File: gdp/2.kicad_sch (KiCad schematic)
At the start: 9 parts, among them IC1 74LS85, IC17 MK3881, IC7 PAL16L8

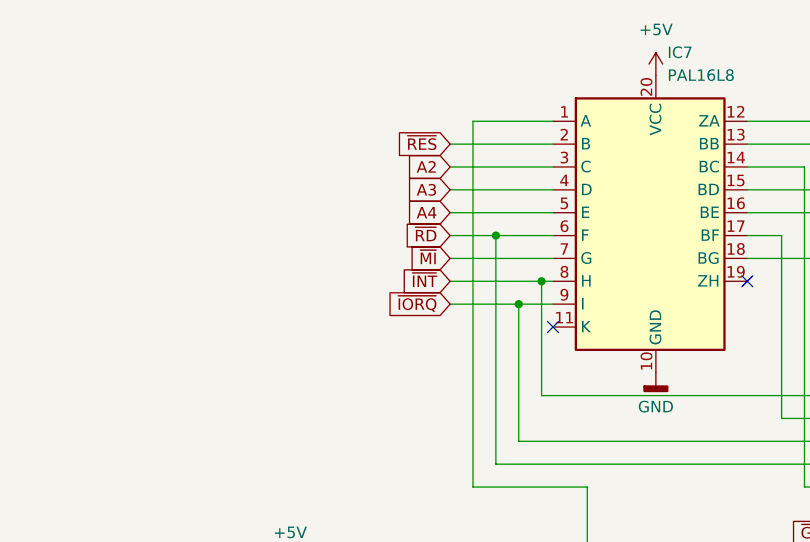
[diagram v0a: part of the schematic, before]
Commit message: Adds Sheet 14 (WIP)
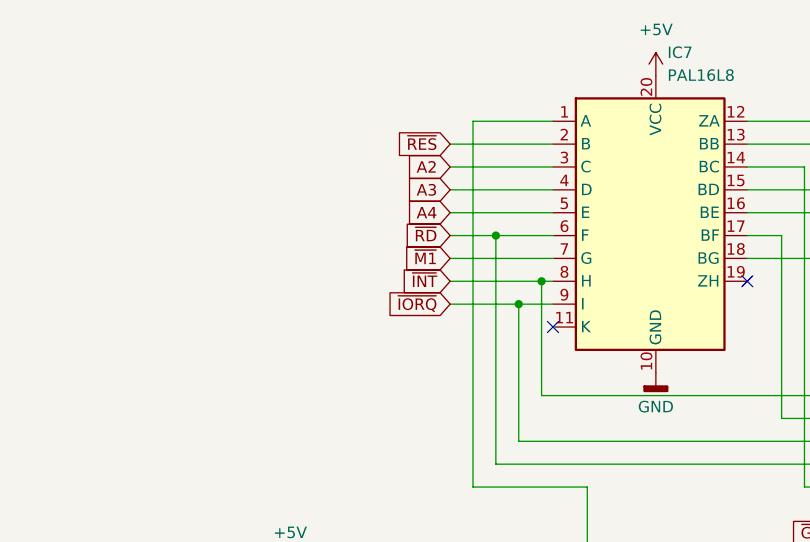
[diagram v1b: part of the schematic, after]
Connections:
- net ~{MI} renamed ~{M1}
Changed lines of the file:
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@@
 		)
 	)
-	(global_label "~{MI}"
+	(global_label "~{M1}"
 		(shape input)
 		(at 115.57 67.31 180)
@@
 		)
 		(property "Intersheetrefs" "${INTERSHEET_REFS}"
-			(at 110.5286 67.31 0)
+			(at 109.9239 67.31 0)
 			(effects
 				(font

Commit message: Initial footprint assignment
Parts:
- IC1: footprint (none) -> Package_DIP:DIP-16_W7.62mm
- IC17: footprint (none) -> Package_DIP:DIP-40_W15.24mm
- IC7: footprint (none) -> Package_DIP:DIP-20_W7.62mm
- R18, R19, R20: footprint (none) -> Resistor_THT:R_Axial_DIN0207_L6.3mm_D2.5mm_P7.62mm_Horizontal
- SH7, SH8, SH9: value SCHALT1 -> SCHALT; footprint (none) -> Connector_PinHeader_2.54mm:PinHeader_1x02_P2.54mm_Vertical
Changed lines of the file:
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@@
 			)
 		)
-		(property "Footprint" ""
+		(property "Footprint" "Resistor_THT:R_Axial_DIN0207_L6.3mm_D2.5mm_P7.62mm_Horizontal"
 			(at 71.12 136.398 90)
 			(effects
@@
 			)
 		)
-		(property "Datasheet" "~"
+		(property "Datasheet" "N/A"
 			(at 71.12 134.62 0)
 			(effects
@@
 			)
 		)
-		(property "Description" ""
+		(property "Description" "N/A"
 			(at 71.12 134.62 0)
 			(effects
@@
 			(project "gdp"
 				(path "/95aff260-2720-4733-a81d-a7a2136fdd14/ed2e3011-1fbf-423e-aa8b-2b4bbe99b1f1"
-					(reference "R18")
+					(reference "R11")
 					(unit 1)
 				)
@@
 		(dnp no)
 		(fields_autoplaced yes)
-		(property "Reference" "#PWR065"
+		(property "Reference" "#PWR032"
 			(at 187.96 144.78 0)
 			(effects
@@
 			(project "gdp"
 				(path "/95aff260-2720-4733-a81d-a7a2136fdd14/ed2e3011-1fbf-423e-aa8b-2b4bbe99b1f1"
-					(reference "#PWR065")
+					(reference "#PWR032")
 					(unit 1)
 				)
@@
 		(dnp no)
 		(fields_autoplaced yes)
-		(property "Reference" "#PWR082"
+		(property "Reference" "#PWR027"
 			(at 114.3 115.57 0)
 			(effects
@@
 			(project "gdp"
 				(path "/95aff260-2720-4733-a81d-a7a2136fdd14/ed2e3011-1fbf-423e-aa8b-2b4bbe99b1f1"
-					(reference "#PWR082")
+					(reference "#PWR027")
 					(unit 1)
 				)
@@
 		(dnp no)
 		(fields_autoplaced yes)
-		(property "Reference" "#PWR064"
+		(property "Reference" "#PWR028"
 			(at 114.3 157.48 0)
 			(effects
@@
 			(project "gdp"
 				(path "/95aff260-2720-4733-a81d-a7a2136fdd14/ed2e3011-1fbf-423e-aa8b-2b4bbe99b1f1"
-					(reference "#PWR064")
+					(reference "#PWR028")
 					(unit 1)
 				)
@@
 			)
 		)
-		(property "Footprint" ""
+		(property "Footprint" "Resistor_THT:R_Axial_DIN0207_L6.3mm_D2.5mm_P7.62mm_Horizontal"
 			(at 71.12 138.938 90)
 			(effects
@@
 			)
 		)
-		(property "Datasheet" "~"
+		(property "Datasheet" "N/A"
 			(at 71.12 137.16 0)
 			(effects
@@
 			)
 		)
-		(property "Description" ""
+		(property "Description" "N/A"
 			(at 71.12 137.16 0)
 			(effects
@@
 			(project "gdp"
 				(path "/95aff260-2720-4733-a81d-a7a2136fdd14/ed2e3011-1fbf-423e-aa8b-2b4bbe99b1f1"
-					(reference "R20")
+					(reference "R12")
 					(unit 1)
 				)
@@
 			)
 		)
-		(property "Footprint" ""
+		(property "Footprint" "Package_DIP:DIP-20_W7.62mm"
 			(at 137.16 41.91 0)
 			(effects
@@
 			)
 		)
-		(property "Datasheet" ""
+		(property "Datasheet" "N/A"
 			(at 137.16 41.91 0)
 			(effects
@@
 			)
 		)
-		(property "Description" ""
+		(property "Description" "N/A"
 			(at 138.43 45.72 0)
 			(effects
@@
 			(project "gdp"
 				(path "/95aff260-2720-4733-a81d-a7a2136fdd14/ed2e3011-1fbf-423e-aa8b-2b4bbe99b1f1"
-					(reference "IC7")
+					(reference "IC5")
 					(unit 1)
 				)
@@
 		(dnp no)
 		(fields_autoplaced yes)
-		(property "Reference" "#PWR074"
+		(property "Reference" "#PWR029"
 			(at 138.43 50.8 0)
 			(effects
@@
 			(project ""
 				(path "/95aff260-2720-4733-a81d-a7a2136fdd14/ed2e3011-1fbf-423e-aa8b-2b4bbe99b1f1"
-					(reference "#PWR074")
+					(reference "#PWR029")
 					(unit 1)
 				)
@@
 			(project "gdp"
 				(path "/95aff260-2720-4733-a81d-a7a2136fdd14/ed2e3011-1fbf-423e-aa8b-2b4bbe99b1f1"
-					(reference "#PWR01")
+					(reference "#PWR025")
 					(unit 1)
 				)
@@
 		(dnp no)
 		(fields_autoplaced yes)
-		(property "Reference" "#PWR063"
+		(property "Reference" "#PWR024"
 			(at 67.31 147.32 0)
 			(effects
@@
 			(project ""
 				(path "/95aff260-2720-4733-a81d-a7a2136fdd14/ed2e3011-1fbf-423e-aa8b-2b4bbe99b1f1"
-					(reference "#PWR063")
+					(reference "#PWR024")
 					(unit 1)
 				)
@@
 		(dnp no)
 		(fields_autoplaced yes)
-		(property "Reference" "#PWR066"
+		(property "Reference" "#PWR030"
 			(at 138.43 86.36 0)
 			(effects
@@
 			(project "gdp"
 				(path "/95aff260-2720-4733-a81d-a7a2136fdd14/ed2e3011-1fbf-423e-aa8b-2b4bbe99b1f1"
-					(reference "#PWR066")
+					(reference "#PWR030")
 					(unit 1)
 				)
@@
 			)
 		)
-		(property "Value" "SCHALT1"
+		(property "Value" "SCHALT"
 			(at 80.01 109.22 0)
 			(effects
@@
 			)
 		)
-		(property "Footprint" ""
+		(property "Footprint" "Connector_PinHeader_2.54mm:PinHeader_1x02_P2.54mm_Vertical"
 			(at 81.28 113.03 0)
 			(effects
@@
 			)
 		)
-		(property "Datasheet" "~"
+		(property "Datasheet" "N/A"
 			(at 81.28 113.03 0)
 			(effects
@@
 			)
 		)
-		(property "Description" ""
+		(property "Description" "N/A"
 			(at 81.28 113.03 0)
 			(effects
@@
 			(project "gdp"
 				(path "/95aff260-2720-4733-a81d-a7a2136fdd14/ed2e3011-1fbf-423e-aa8b-2b4bbe99b1f1"
-					(reference "SH8")
+					(reference "SH5")
 					(unit 1)
 				)
@@
 		(dnp no)
 		(fields_autoplaced yes)
-		(property "Reference" "#PWR075"
+		(property "Reference" "#PWR031"
 			(at 187.96 83.82 0)
 			(effects
@@
 			(project ""
 				(path "/95aff260-2720-4733-a81d-a7a2136fdd14/ed2e3011-1fbf-423e-aa8b-2b4bbe99b1f1"
-					(reference "#PWR075")
+					(reference "#PWR031")
 					(unit 1)
 				)
@@
 			)
 		)
-		(property "Value" "SCHALT1"
+		(property "Value" "SCHALT"
 			(at 77.47 109.22 0)
 			(effects
@@
 			)
 		)
-		(property "Footprint" ""
+		(property "Footprint" "Connector_PinHeader_2.54mm:PinHeader_1x02_P2.54mm_Vertical"
 			(at 78.74 113.03 0)
 			(effects
@@
 			)
 		)
-		(property "Datasheet" "~"
+		(property "Datasheet" "N/A"
 			(at 78.74 113.03 0)
 			(effects
@@
 			)
 		)
-		(property "Description" ""
+		(property "Description" "N/A"
 			(at 78.74 113.03 0)
 			(effects
@@
 			(project "gdp"
 				(path "/95aff260-2720-4733-a81d-a7a2136fdd14/ed2e3011-1fbf-423e-aa8b-2b4bbe99b1f1"
-					(reference "SH7")
+					(reference "SH4")
 					(unit 1)
 				)
@@
 			)
 		)
-		(property "Value" "SCHALT1"
+		(property "Value" "SCHALT"
 			(at 82.55 109.22 0)
 			(effects
@@
 			)
 		)
-		(property "Footprint" ""
+		(property "Footprint" "Connector_PinHeader_2.54mm:PinHeader_1x02_P2.54mm_Vertical"
 			(at 83.82 113.03 0)
 			(effects
@@
 			)
 		)
-		(property "Datasheet" "~"
+		(property "Datasheet" "N/A"
 			(at 83.82 113.03 0)
 			(effects
@@
 			)
 		)
-		(property "Description" ""
+		(property "Description" "N/A"
 			(at 83.82 113.03 0)
 			(effects
@@
 			(project "gdp"
 				(path "/95aff260-2720-4733-a81d-a7a2136fdd14/ed2e3011-1fbf-423e-aa8b-2b4bbe99b1f1"
-					(reference "SH9")
+					(reference "SH6")
 					(unit 1)
 				)
@@
 		(dnp no)
 		(fields_autoplaced yes)
-		(property "Reference" "#PWR081"
+		(property "Reference" "#PWR026"
 			(at 97.79 125.73 0)
 			(effects
@@
 			(project "gdp"
 				(path "/95aff260-2720-4733-a81d-a7a2136fdd14/ed2e3011-1fbf-423e-aa8b-2b4bbe99b1f1"
-					(reference "#PWR081")
+					(reference "#PWR026")
 					(unit 1)
 				)
@@
 			)
 		)
-		(property "Footprint" ""
+		(property "Footprint" "Package_DIP:DIP-40_W15.24mm"
 			(at 186.69 77.47 0)
 			(effects
@@
 			)
 		)
-		(property "Datasheet" ""
+		(property "Datasheet" "N/A"
 			(at 186.69 77.47 0)
 			(effects
@@
 			)
 		)
-		(property "Description" ""
+		(property "Description" "N/A"
 			(at 182.88 77.47 0)
 			(effects
@@
 			(project "gdp"
 				(path "/95aff260-2720-4733-a81d-a7a2136fdd14/ed2e3011-1fbf-423e-aa8b-2b4bbe99b1f1"
-					(reference "IC17")
+					(reference "IC6")
 					(unit 1)
 				)
@@
 			)
 		)
-		(property "Footprint" ""
+		(property "Footprint" "Package_DIP:DIP-16_W7.62mm"
 			(at 116.84 109.22 0)
 			(effects
@@
 			)
 		)
-		(property "Datasheet" ""
+		(property "Datasheet" "N/A"
 			(at 116.84 109.22 0)
 			(effects
@@
 			)
 		)
-		(property "Description" ""
+		(property "Description" "N/A"
 			(at 110.49 118.11 0)
 			(effects
@@
 			(project "gdp"
 				(path "/95aff260-2720-4733-a81d-a7a2136fdd14/ed2e3011-1fbf-423e-aa8b-2b4bbe99b1f1"
-					(reference "IC6")
+					(reference "IC4")
 					(unit 1)
 				)
@@
 			)
 		)
-		(property "Footprint" ""
+		(property "Footprint" "Resistor_THT:R_Axial_DIN0207_L6.3mm_D2.5mm_P7.62mm_Horizontal"
 			(at 71.12 133.858 90)
 			(effects
@@
 			)
 		)
-		(property "Datasheet" "~"
+		(property "Datasheet" "N/A"
 			(at 71.12 132.08 0)
 			(effects
@@
 			)
 		)
-		(property "Description" ""
+		(property "Description" "N/A"
 			(at 71.12 132.08 0)
 			(effects
@@
 			(project "gdp"
 				(path "/95aff260-2720-4733-a81d-a7a2136fdd14/ed2e3011-1fbf-423e-aa8b-2b4bbe99b1f1"
-					(reference "R19")
-					(unit 1)
-				)
+					(reference "R10")
+					(unit 1)
+				)
